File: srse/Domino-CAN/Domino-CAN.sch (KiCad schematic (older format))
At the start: 4 parts, among them P1 UART, U1 DOMINO_CORE, U2 PIC18F25K80, U3 FT230XS

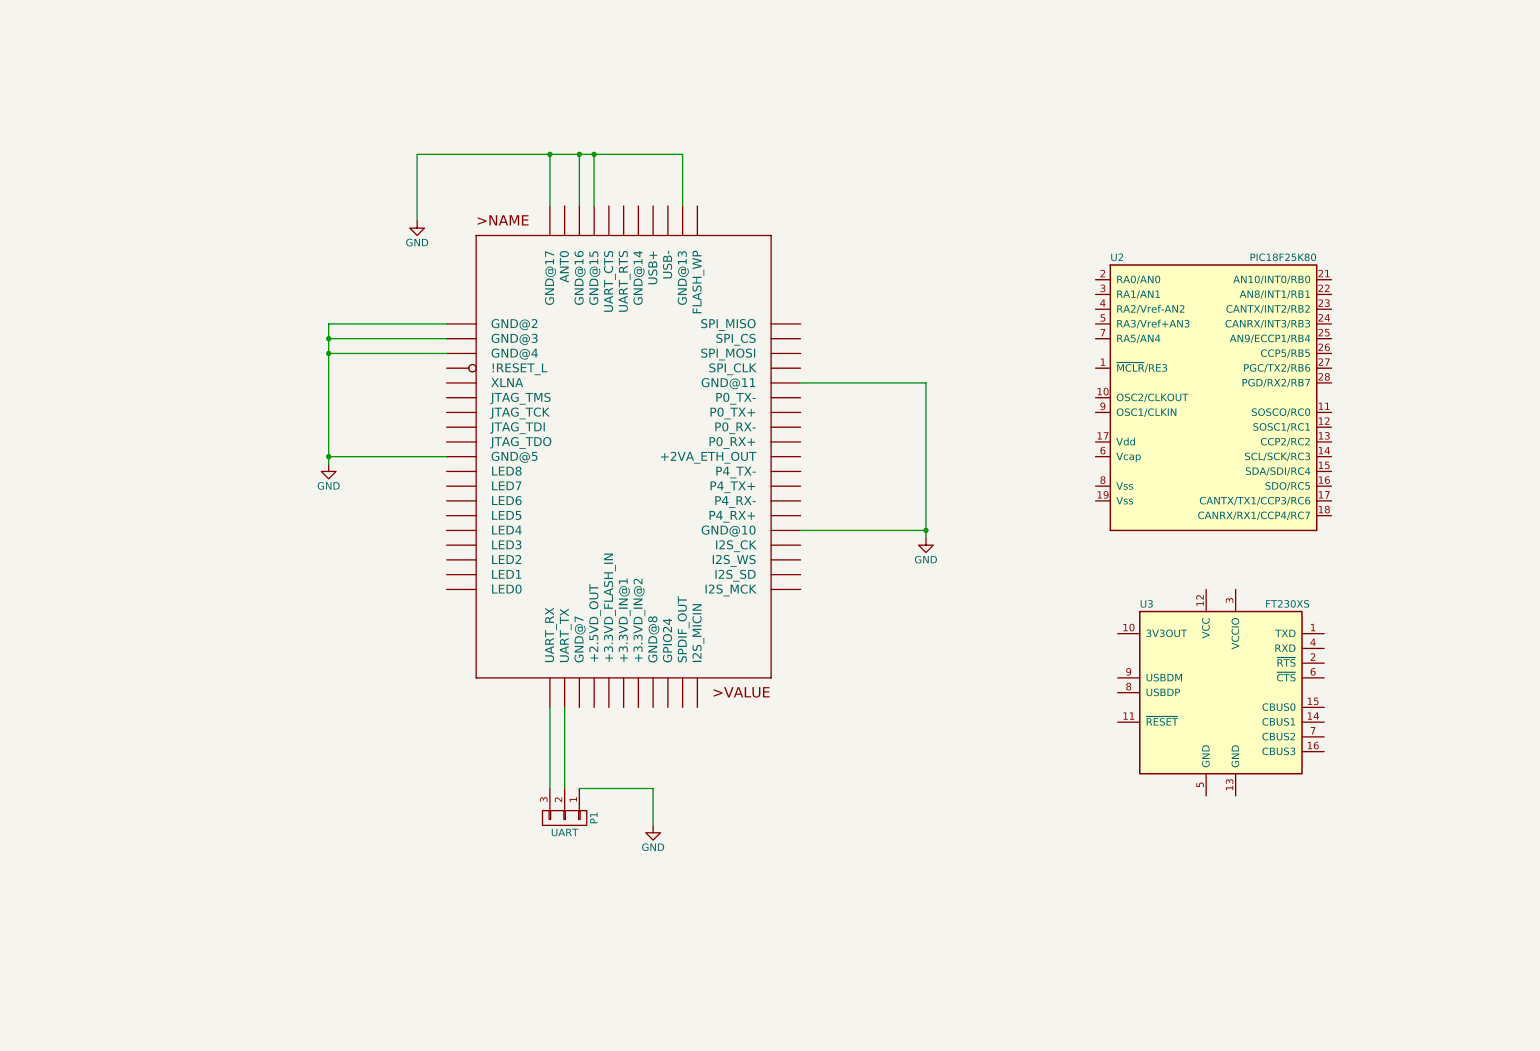
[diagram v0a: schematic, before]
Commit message: wip
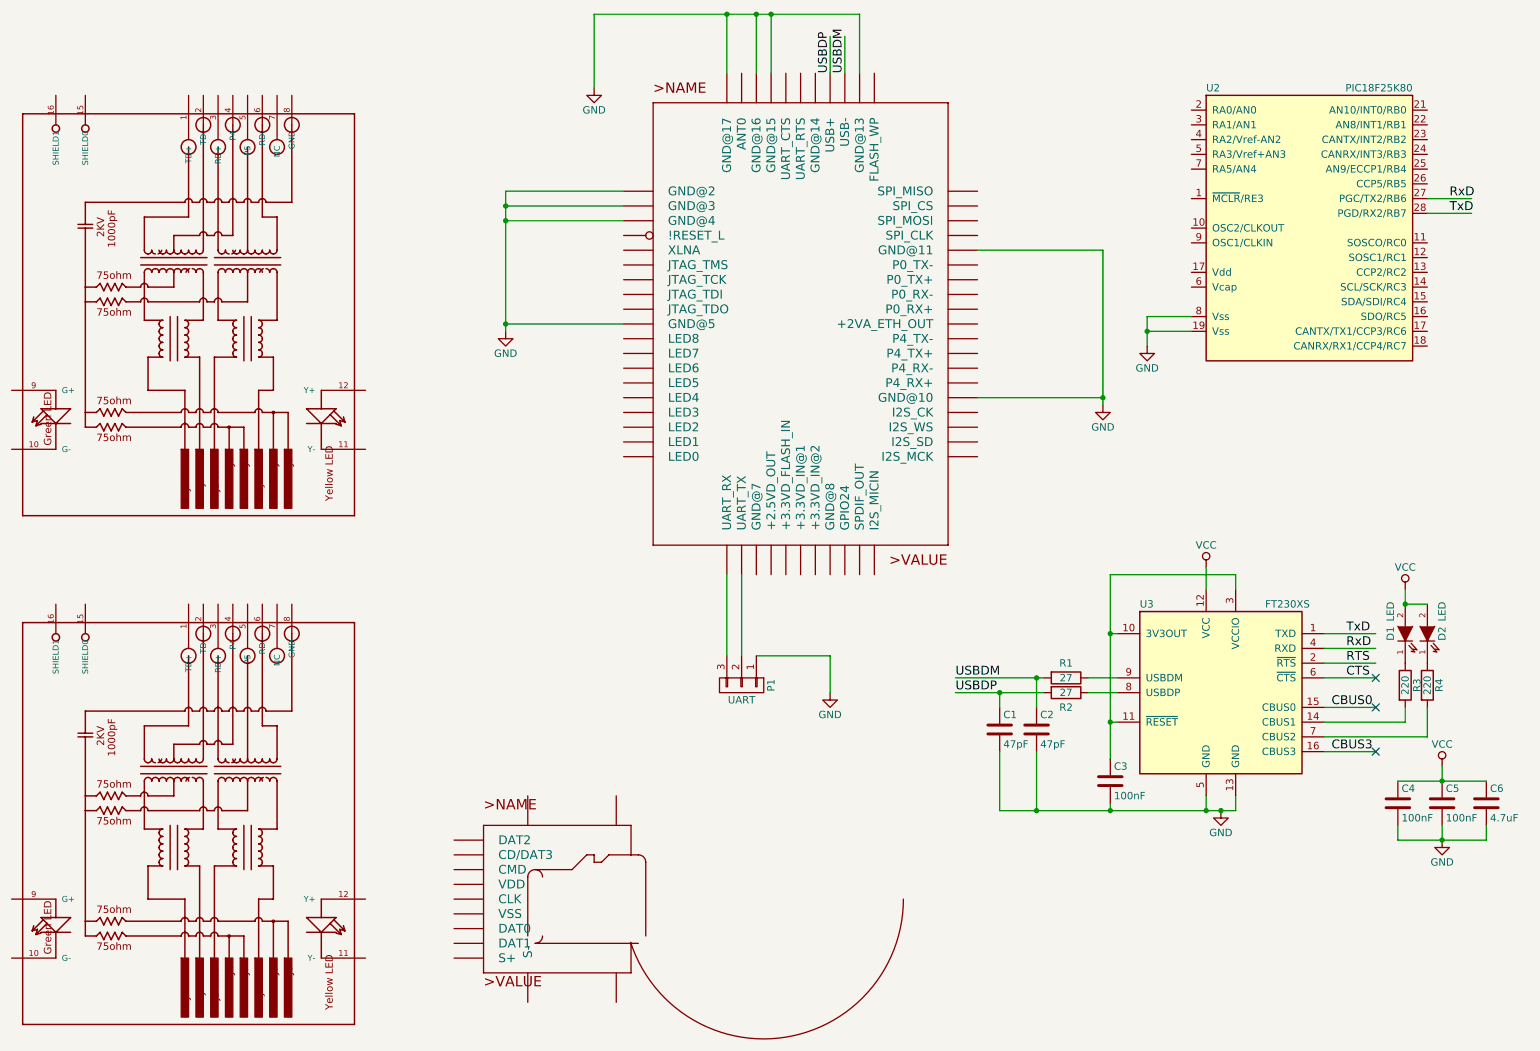
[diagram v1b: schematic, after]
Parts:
- added C1, C2: 47pF, Resistors_SMD:R_0805_HandSoldering_II, symbol C
- added C3: 100nF, symbol C
- added C4, C5: 100nF, Resistors_SMD:R_0805_HandSoldering_II, symbol C
- added C6: 4.7uF, Resistors_SMD:R_0805_HandSoldering_II, symbol C
- added D1, D2: LED, symbol LED
- added R1, R2: 27, Resistors_SMD:R_0805_HandSoldering_II, symbol R
- added R3, R4: 220, Resistors_SMD:R_0805_HandSoldering_II, symbol R
- added U4, U5: HR911105A, RJ45ALED_1PRIMARY, symbol HR911105A
- added U6: MICRO-SD_SD-007, symbol MICRO-SD_SD-007
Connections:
- net labels added: CBUS0, CBUS3, CTS, RTS, RxD, TxD, USBDM, USBDP, VCC
- wire segments 18 -> 61
- no-connect marks 0 -> 3
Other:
- moved on the sheet: P1, U2

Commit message: wip
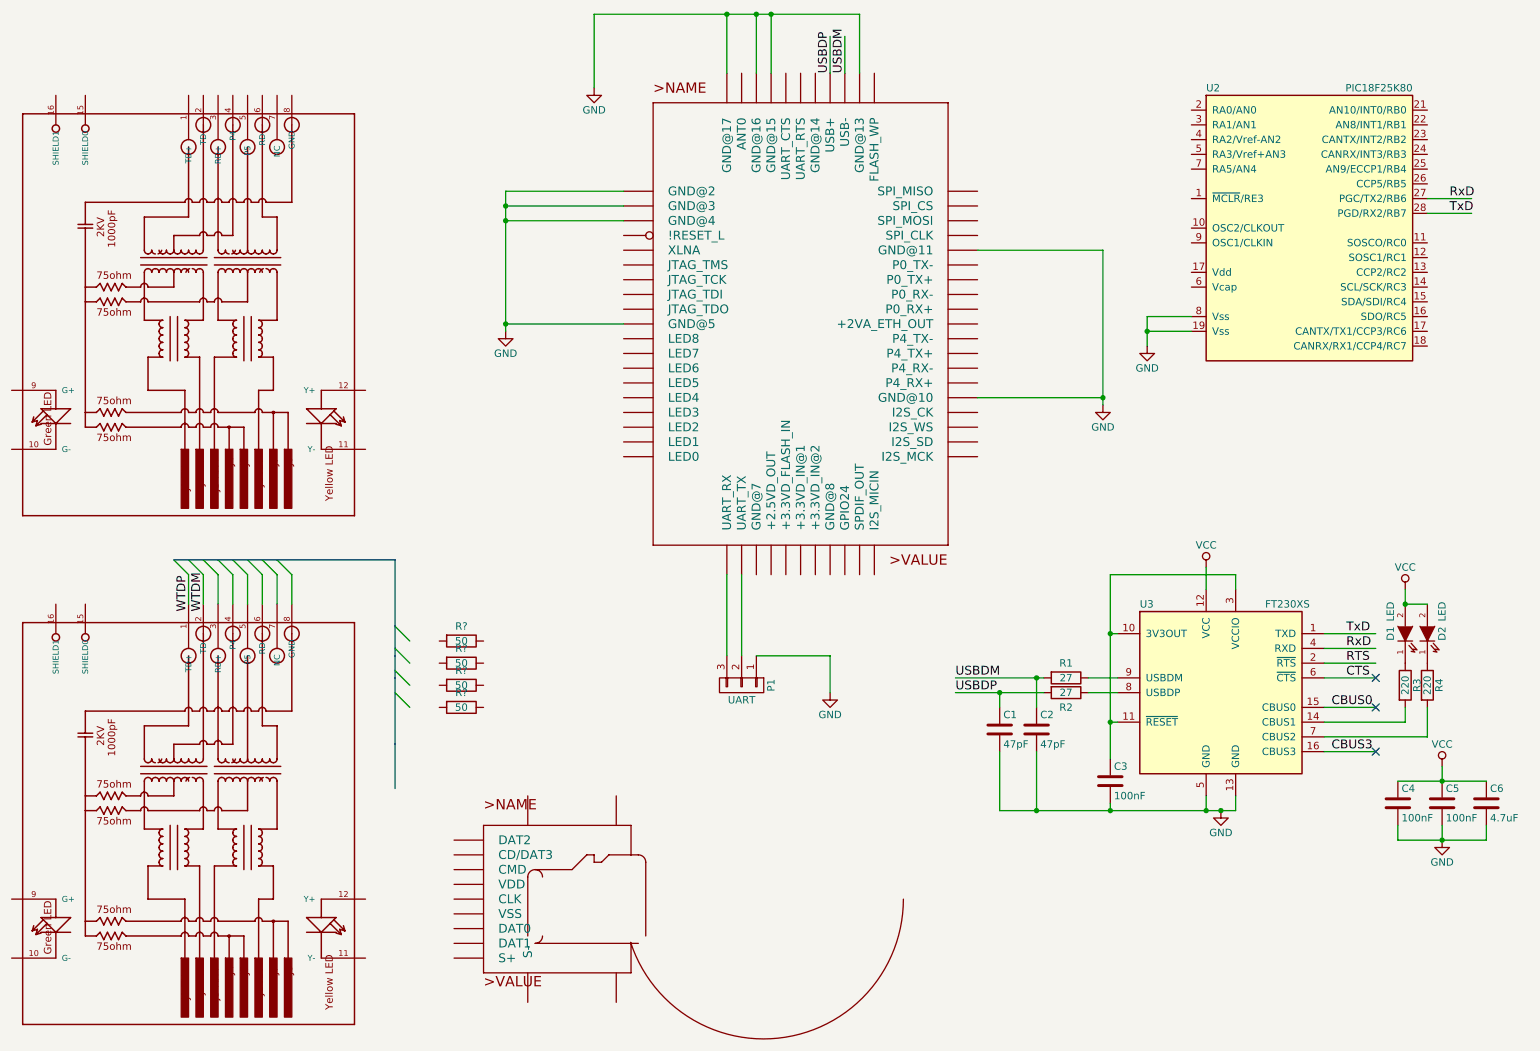
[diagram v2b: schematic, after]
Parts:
- added R? (x4): 50, Resistors_SMD:R_0805_HandSoldering_II, symbol R
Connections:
- net labels added: WTDM, WTDP
- wire segments 61 -> 87
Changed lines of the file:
@@
 LIBS:contrib
 LIBS:valves
-LIBS:Domino
 LIBS:microchip_pic18mcu
 LIBS:ftdi
-LIBS:HR911105A
 LIBS:Domino-CAN-cache
 EELAYER 25 0
@@
 	4100 2100 4900 2100
 Wire Wire Line
-	4100 1900 4100 2850
+	4100 1900 4100 2000
+Wire Wire Line
+	4100 2000 4100 2100
+Wire Wire Line
+	4100 2100 4100 2800
+Wire Wire Line
+	4100 2800 4100 2850
 Wire Wire Line
 	4900 2000 4100 2000
@@
 	5600 1100 5600 700
 Wire Wire Line
-	4700 700  6500 700
+	4700 700  5600 700
+Wire Wire Line
+	5600 700  5800 700
+Wire Wire Line
+	5800 700  5900 700
+Wire Wire Line
+	5900 700  6500 700
 Wire Wire Line
 	4700 700  4700 1200
@@
 	7300 3300 8150 3300
 Wire Wire Line
-	8150 2300 8150 3350
+	8150 2300 8150 3300
+Wire Wire Line
+	8150 3300 8150 3350
 Wire Wire Line
 	7300 2300 8150 2300
@@
 	8750 2850 8450 2850
 Wire Wire Line
-	8450 2750 8450 2950
+	8450 2750 8450 2850
+Wire Wire Line
+	8450 2850 8450 2950
 Wire Wire Line
 	8750 2750 8450 2750
@@
 	8850 6100 8850 6000
 Wire Wire Line
-	7450 6100 9050 6100
+	7450 6100 7700 6100
+Wire Wire Line
+	7700 6100 8200 6100
+Wire Wire Line
+	8200 6100 8850 6100
+Wire Wire Line
+	8850 6100 8950 6100
+Wire Wire Line
+	8950 6100 9050 6100
 Wire Wire Line
 	9050 6100 9050 6000
@@
 	9050 4500 8200 4500
 Wire Wire Line
-	8200 4500 8200 5750
+	8200 4500 8200 4900
+Wire Wire Line
+	8200 4900 8200 5500
+Wire Wire Line
+	8200 5500 8200 5750
 Wire Wire Line
 	8200 4900 8250 4900
@@
 Connection ~ 8200 5500
 Wire Wire Line
-	7150 5200 7750 5200
-Wire Wire Line
-	7150 5300 7750 5300
+	7150 5200 7700 5200
+Wire Wire Line
+	7700 5200 7750 5200
+Wire Wire Line
+	7150 5300 7450 5300
+Wire Wire Line
+	7450 5300 7750 5300
 Wire Wire Line
 	7450 5400 7450 5300
@@
 Connection ~ 7700 6100
 Wire Wire Line
-	10150 5900 10750 5900
+	10150 5900 10450 5900
+Wire Wire Line
+	10450 5900 10750 5900
 Connection ~ 10450 5900
 Wire Wire Line
@@
 	10150 6200 10150 6300
 Wire Wire Line
-	10150 6300 10750 6300
+	10150 6300 10450 6300
+Wire Wire Line
+	10450 6300 10750 6300
 Wire Wire Line
 	10750 6300 10750 6200
@@
 U 1 1 56BA5AED
 P 4450 6700
-F 0 "U6" H 4450 6700 0   0001 C CNN
+F 0 "U6" H 4450 6700 60  0001 C CNN
 F 1 "MICRO-SD_SD-007" H 4450 6700 10  0001 C CNN
 F 2 "" H 4450 6700 60  0000 C CNN
@@
 	1    0    0    -1
 $EndComp
+$Comp
+L R R?
+U 1 1 56BA394D
+P 3800 4950
+F 0 "R?" V 3700 4950 50  0000 C CNN
+F 1 "50" V 3800 4950 50  0000 C CNN
+F 2 "Resistors_SMD:R_0805_HandSoldering_II" H 3730 4950 50  0001 C CNN
+F 3 "" H 3800 4950 50  0000 C CNN
+	1    3800 4950
+	0    1    1    0
+$EndComp
+$Comp
+L R R?
+U 1 1 56BA3AE8
+P 3800 5100
+F 0 "R?" V 3700 5100 50  0000 C CNN
+F 1 "50" V 3800 5100 50  0000 C CNN
+F 2 "Resistors_SMD:R_0805_HandSoldering_II" H 3730 5100 50  0001 C CNN
+F 3 "" H 3800 5100 50  0000 C CNN
+	1    3800 5100
+	0    1    1    0
+$EndComp
+$Comp
+L R R?
+U 1 1 56BA3B32
+P 3800 5250
+F 0 "R?" V 3700 5250 50  0000 C CNN
+F 1 "50" V 3800 5250 50  0000 C CNN
+F 2 "Resistors_SMD:R_0805_HandSoldering_II" H 3730 5250 50  0001 C CNN
+F 3 "" H 3800 5250 50  0000 C CNN
+	1    3800 5250
+	0    1    1    0
+$EndComp
+$Comp
+L R R?
+U 1 1 56BA3B7D
+P 3800 5400
+F 0 "R?" V 3700 5400 50  0000 C CNN
+F 1 "50" V 3800 5400 50  0000 C CNN
+F 2 "Resistors_SMD:R_0805_HandSoldering_II" H 3730 5400 50  0001 C CNN
+F 3 "" H 3800 5400 50  0000 C CNN
+	1    3800 5400
+	0    1    1    0
+$EndComp
+Wire Bus Line
+	3350 4400 3350 4850
+Wire Bus Line
+	3350 4850 3350 5050
+Wire Bus Line
+	3350 5050 3350 5200
+Wire Bus Line
+	3350 5200 3350 5650
+Wire Bus Line
+	3350 5650 3350 5950
+Entry Wire Line
+	3350 4850 3450 4950
+Entry Wire Line
+	3350 5000 3450 5100
+Entry Wire Line
+	3350 5150 3450 5250
+Entry Wire Line
+	3350 5300 3450 5400
+Wire Wire Line
+	1950 4700 1950 4500
+Wire Wire Line
+	2050 4700 2050 4500
+Wire Wire Line
+	2150 4500 2150 4700
+Wire Wire Line
+	2250 4700 2250 4500
+Wire Wire Line
+	2350 4700 2350 4500
+Wire Wire Line
+	2450 4700 2450 4500
+Wire Wire Line
+	2550 4700 2550 4500
+Wire Wire Line
+	2650 4700 2650 4500
+Wire Bus Line
+	1850 4400 1950 4400
+Wire Bus Line
+	1950 4400 2050 4400
+Wire Bus Line
+	2050 4400 2150 4400
+Wire Bus Line
+	2150 4400 2250 4400
+Wire Bus Line
+	2250 4400 2350 4400
+Wire Bus Line
+	2350 4400 2450 4400
+Wire Bus Line
+	2450 4400 2550 4400
+Wire Bus Line
+	2550 4400 3350 4400
+Entry Wire Line
+	2050 4400 2150 4500
+Entry Wire Line
+	1950 4400 2050 4500
+Entry Wire Line
+	1850 4400 1950 4500
+Entry Wire Line
+	2150 4400 2250 4500
+Entry Wire Line
+	2250 4400 2350 4500
+Entry Wire Line
+	2350 4400 2450 4500
+Entry Wire Line
+	2450 4400 2550 4500
+Entry Wire Line
+	2550 4400 2650 4500
+Text Label 1950 4750 1    60   ~ 0
+WTDP
+Text Label 2050 4750 1    60   ~ 0
+WTDM
 $EndSCHEMATC
